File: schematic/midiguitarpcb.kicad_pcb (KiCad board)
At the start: 2 copper layers, 50 x 50 mm, 34 parts, among them CN1 NMJ6HCD2, J1 USB_C_Receptacle_USB2.0_16P, SW1 SW_Omron_B3FS, U1 AMS1117-3.3, U2 DIN-504D-M5, U3 STM32H743ZITx

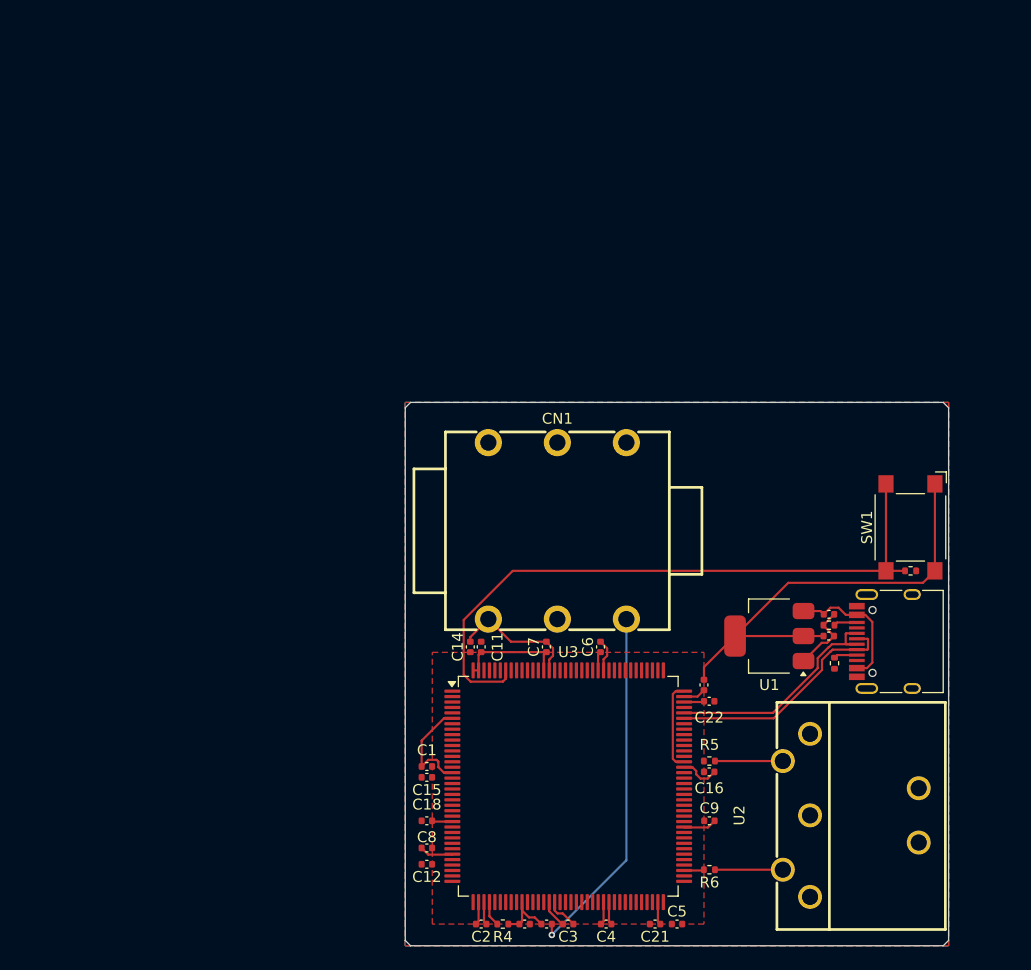
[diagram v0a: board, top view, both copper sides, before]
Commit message: redo pcb
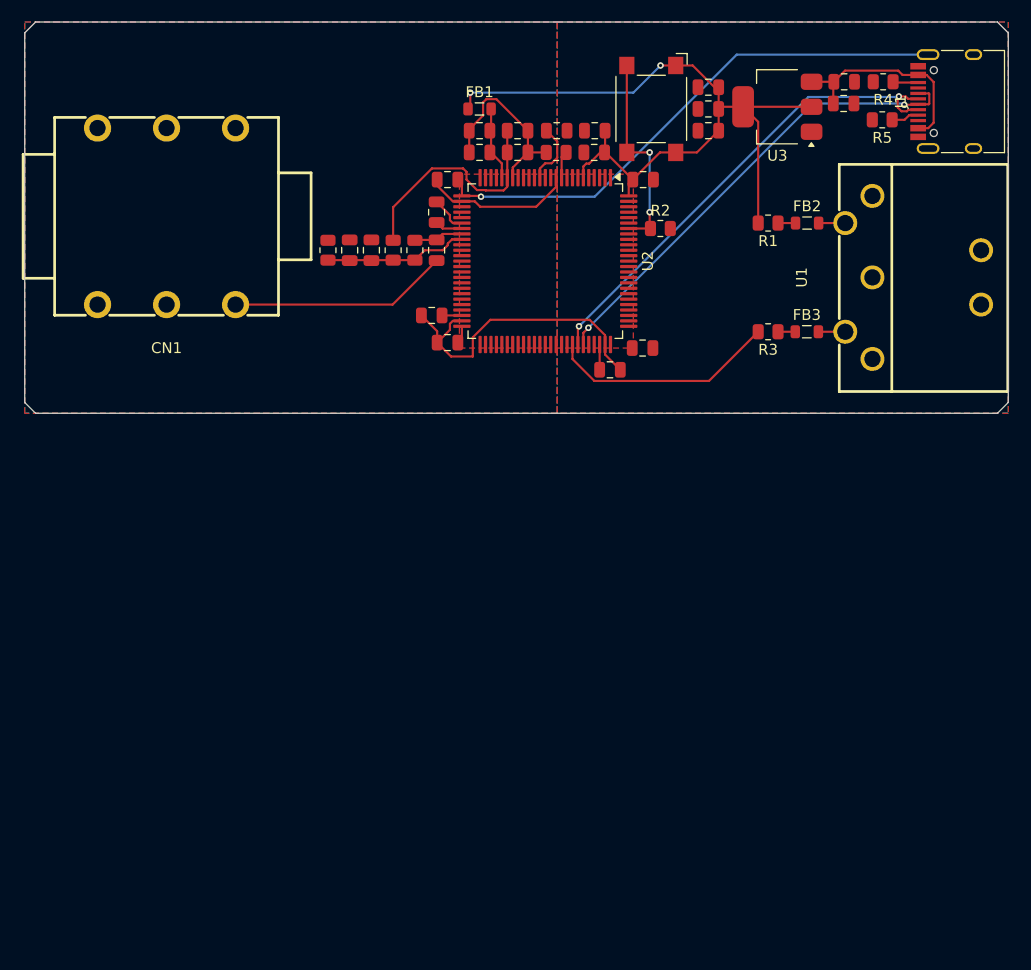
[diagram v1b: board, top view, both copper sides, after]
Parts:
- added FB1: FerriteBead, Inductor_SMD:L_0805_2012Metric, F.Cu at (56.9, 23.0)
- added FB2: FerriteBead, Inductor_SMD:L_0805_2012Metric, F.Cu at (87.0, 33.5)
- added FB3: FerriteBead, Inductor_SMD:L_0805_2012Metric, F.Cu at (87.0, 43.5)
- added R7: 100K, Resistor_SMD:R_0805_2012Metric, F.Cu at (42.9, 36.0)
- added R8: 100K, Resistor_SMD:R_0805_2012Metric, F.Cu at (50.9, 36.0)
- added R9: 0, Resistor_SMD:R_0805_2012Metric, F.Cu at (63.9, 27.0)
- C1, C4, C9: value 100nF -> 1uF; footprint Capacitor_SMD:C_0402_1005Metric -> Capacitor_SMD:C_0805_2012Metric
- C10: value 100nF -> 10uF; footprint Capacitor_SMD:C_0402_1005Metric -> Capacitor_SMD:C_0805_2012Metric
- C11: value 100nF -> 100pF; footprint Capacitor_SMD:C_0402_1005Metric -> Capacitor_SMD:C_0805_2012Metric
- C12: value 4.7uF -> 100nF; footprint Capacitor_SMD:C_0402_1005Metric -> Capacitor_SMD:C_0805_2012Metric
- C13: value 10uF -> 1uF; footprint Capacitor_SMD:C_0402_1005Metric -> Capacitor_SMD:C_0805_2012Metric
- C14, C16: value 100nF -> 2.2uF; footprint Capacitor_SMD:C_0402_1005Metric -> Capacitor_SMD:C_0805_2012Metric
- C15, C18, C2, C3, C5, C6, C7: footprint Capacitor_SMD:C_0402_1005Metric -> Capacitor_SMD:C_0805_2012Metric
- C17: value 10uF -> 100nF; footprint Capacitor_SMD:C_0402_1005Metric -> Capacitor_SMD:C_0805_2012Metric
- C19: value 1uF -> 100nF; footprint Capacitor_SMD:C_0402_1005Metric -> Capacitor_SMD:C_0805_2012Metric
- C20: value 100pF -> 100nF; footprint Capacitor_SMD:C_0402_1005Metric -> Capacitor_SMD:C_0805_2012Metric
- C21: value 2.2uF -> 100nF; footprint Capacitor_SMD:C_0402_1005Metric -> Capacitor_SMD:C_0805_2012Metric
- C22: value 2.2uF -> 4.7uF; footprint Capacitor_SMD:C_0402_1005Metric -> Capacitor_SMD:C_0805_2012Metric
- C8: value 1uF -> 10uF; footprint Capacitor_SMD:C_0402_1005Metric -> Capacitor_SMD:C_0805_2012Metric
- R1: value 10K -> 33; footprint Resistor_SMD:R_0402_1005Metric -> Resistor_SMD:R_0805_2012Metric
- R2: value 5.1K -> 10K; footprint Resistor_SMD:R_0402_1005Metric -> Resistor_SMD:R_0805_2012Metric
- R3: value 5.1K -> 10; footprint Resistor_SMD:R_0402_1005Metric -> Resistor_SMD:R_0805_2012Metric
- R4: value 100K -> 5.1K; footprint Resistor_SMD:R_0402_1005Metric -> Resistor_SMD:R_0805_2012Metric
- R5: value 33 -> 5.1K; footprint Resistor_SMD:R_0402_1005Metric -> Resistor_SMD:R_0805_2012Metric
- R6: value 10 -> 100K; footprint Resistor_SMD:R_0402_1005Metric -> Resistor_SMD:R_0805_2012Metric
- U1: value AMS1117-3.3 -> DIN-504D-M5; footprint Package_TO_SOT_SMD:SOT-223-3_TabPin2 -> din5:CONN-TH_DIN-504D-M5
- U2: value DIN-504D-M5 -> STM32H743VGTx; footprint din5:CONN-TH_DIN-504D-M5 -> Package_QFP:LQFP-100_14x14mm_P0.5mm
- U3: value STM32H743ZITx -> AMS1117-3.3; footprint Package_QFP:LQFP-144_20x20mm_P0.5mm -> Package_TO_SOT_SMD:SOT-223-3_TabPin2
- moved R4 85.0 mm to (94.0, 20.5)
- moved C8 78.5 mm to (90.3, 22.5), turned to 0 degrees
- moved C12 74.2 mm to (77.9, 23.0)
- moved C4 73.5 mm to (60.4, 25.0), turned to 0 degrees
- moved C3 73.0 mm to (64.0, 25.0)
- moved C5 72.5 mm to (60.4, 27.0)
- moved C21 71.2 mm to (67.4, 27.0)
- moved C2 71.0 mm to (56.9, 27.0)
- moved C20 69.4 mm to (71.9, 29.5), turned to 0 degrees
- moved C19 69.1 mm to (53.9, 29.5)
- moved U3 65.4 mm to (84.2, 22.8), turned to 180 degrees
- moved R6 64.0 mm to (48.9, 36.0), turned to -90 degrees
- moved C9 62.1 mm to (44.9, 36.0), turned to 90 degrees
- moved R5 61.1 mm to (93.9, 24.0)
- moved C1 58.7 mm to (56.9, 25.0)
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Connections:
- C1 pad 1: +3V3 -> Net-(U2-VDDA)
- C1 pad 2: GND -> GNDA
- C11 pad 1: +3V3 -> Net-(U2-PC4)
- C11 pad 2: GND -> Net-(U2-PA7)
- C13 pad 1: VBUS -> Net-(CN1-T)
- C13 pad 2: GND -> Net-(U2-PC5)
- C14 pad 1: +3V3 -> Net-(C14-Pad1)
- C16 pad 1: +3V3 -> Net-(C16-Pad1)
- C18 pad 1: Net-(U3-NRST) -> +3V3
- C19 pad 1: Net-(U3-PB0) -> +3V3
- C19 pad 2: Net-(CN1-T) -> GND
- C2 pad 1: +3V3 -> Net-(U2-VDDA)
- C2 pad 2: GND -> GNDA
- C20 pad 1: GND -> +3V3
- C20 pad 2: Net-(U3-PB0) -> GND
- C21 pad 1: Net-(C21-Pad1) -> +3V3
- C22 pad 1: Net-(C22-Pad1) -> +3V3
- C3 pad 1: +3V3 -> GND
- C3 pad 2: GND -> Net-(U2-NRST)
- C4 pad 1: +3V3 -> VDDA
- C4 pad 2: GND -> GNDA
- C5 pad 1: +3V3 -> VDDA
- C5 pad 2: GND -> GNDA
- C6 pad 1: +3V3 -> Net-(U3-VI)
- C7 pad 1: +3V3 -> Net-(U2-PB0)
- C7 pad 2: GND -> GNDA
- C8 pad 1: +3V3 -> Net-(U3-VI)
- C9 pad 1: +3V3 -> Net-(U2-PB0)
- C9 pad 2: GND -> GNDA
- CN1 pad 3: GND -> GNDA
- CN1 pad 4: GND -> GNDA
- J1 pad A4: VBUS -> Net-(U3-VI)
- J1 pad A6: Net-(U3-PA12) -> Net-(U2-PA11)
- J1 pad A7: Net-(U3-PA11) -> Net-(U2-PA10)
- J1 pad A9: VBUS -> Net-(U3-VI)
- J1 pad B4: VBUS -> Net-(U3-VI)
- J1 pad B6: Net-(U3-PA12) -> Net-(U2-PA11)
- J1 pad B7: Net-(U3-PA11) -> Net-(U2-PA10)
- J1 pad B9: VBUS -> Net-(U3-VI)
- R1 pad 1: Net-(U3-BOOT0) -> Net-(FB2-Pad1)
- R1 pad 2: GND -> +3V3
- R2 pad 1: Net-(J1-CC2) -> Net-(U2-BOOT0)
- R3 pad 1: Net-(J1-CC1) -> Net-(FB3-Pad1)
- R3 pad 2: GND -> Net-(U2-PA9)
- R4 pad 1: Net-(U3-PB0) -> Net-(J1-CC2)
- R4 pad 2: Net-(U3-PA4) -> GND
- R5 pad 1: Net-(R5-Pad1) -> Net-(J1-CC1)
- R5 pad 2: +3V3 -> GND
- R6 pad 1: Net-(R6-Pad1) -> VDDA
- R6 pad 2: Net-(U3-PB14) -> Net-(U2-PB0)
- SW1 pad 2: Net-(U3-BOOT0) -> Net-(U2-BOOT0)
- U1 pad 1: GND -> unconnected-(U1-Pad1)
- U1 pad 2: +3V3 -> GND
- U1 pad 3: VBUS -> unconnected-(U1-Pad3)
- U2 pad 2: GND -> unconnected-(U2-PE3-Pad2)
- U2 pad 4: Net-(R5-Pad1) -> unconnected-(U2-PE5-Pad4)
- U2 pad 5: Net-(R6-Pad1) -> unconnected-(U2-PE6-Pad5)
- U2 pad 6: GND -> +3V3
- U2 pad 7: GND -> unconnected-(U2-PC13-Pad7)
- U3 pad 1: unconnected-(U3-PE2-Pad1) -> GND
- U3 pad 2: unconnected-(U3-PE3-Pad2) -> +3V3
- U3 pad 3: unconnected-(U3-PE4-Pad3) -> Net-(U3-VI)
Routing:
- net Net-(U3-BOOT0): track 60.5 -> 0.00 mm
- net Net-(U2-PA10): track 0.00 -> 44.9 mm, vias 0 -> 2
- net Net-(U2-PA11): track 0.00 -> 43.7 mm, vias 0 -> 2
- net GND: track 50.2 -> 81.8 mm, vias 0 -> 1
- net Net-(U3-PA11): track 22.0 -> 0.00 mm
- net Net-(U3-PA12): track 22.0 -> 0.00 mm
- net VDDA: track 0.00 -> 21.6 mm
- net Net-(U2-PA9): track 0.00 -> 21.1 mm
- net Net-(U3-VI): track 0.00 -> 19.5 mm
- net Net-(U2-BOOT0): track 0.00 -> 19.1 mm, vias 0 -> 2
- net GNDA: track 0.00 -> 17.2 mm
- net +3V3: track 69.5 -> 85.9 mm, vias 0 -> 2
- net Net-(U2-PB0): track 0.00 -> 13.2 mm
- net Net-(CN1-T): track 32.9 -> 20.2 mm, vias 1 -> 0
- net VBUS: track 12.6 -> 0.00 mm
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- added copper zone on B.Cu, net GNDA
- added copper zone on F.Cu, net GNDA
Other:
- board size 50 x 50 mm -> 90.5 x 36 mm
